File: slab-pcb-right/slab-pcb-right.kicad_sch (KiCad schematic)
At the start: 125 parts, among them J1 MagnetR, J2 MagnetL, J3 TRRS_R, J4 TRRS_L, J5 SSD1306, J6 Conn_01x06, Q1 MMBT3906, SW1 RotaryEncoder, U1 Seeeduino Xiao rp2040, U2 PCA9555PW, U3 PCA9555PW, U4 ADS1110, U5 SN74AHCT125PWR

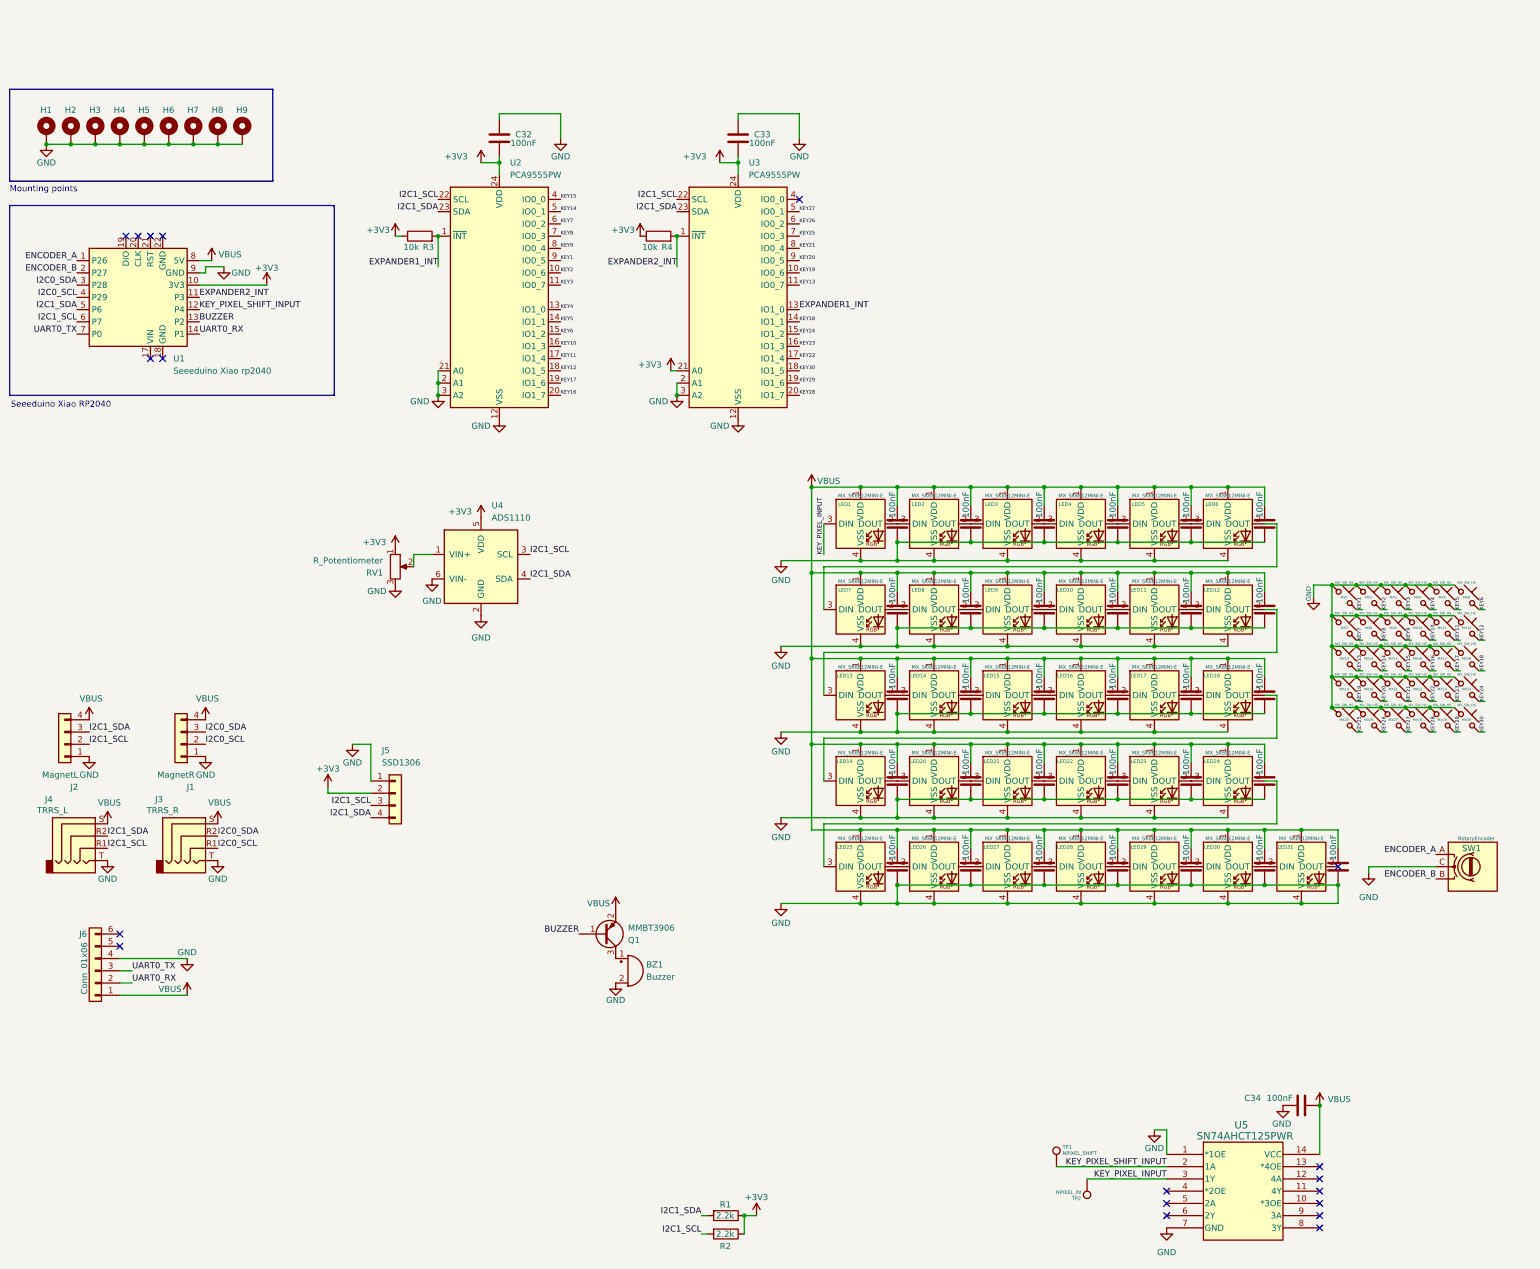
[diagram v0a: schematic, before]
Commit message: feat: start right board
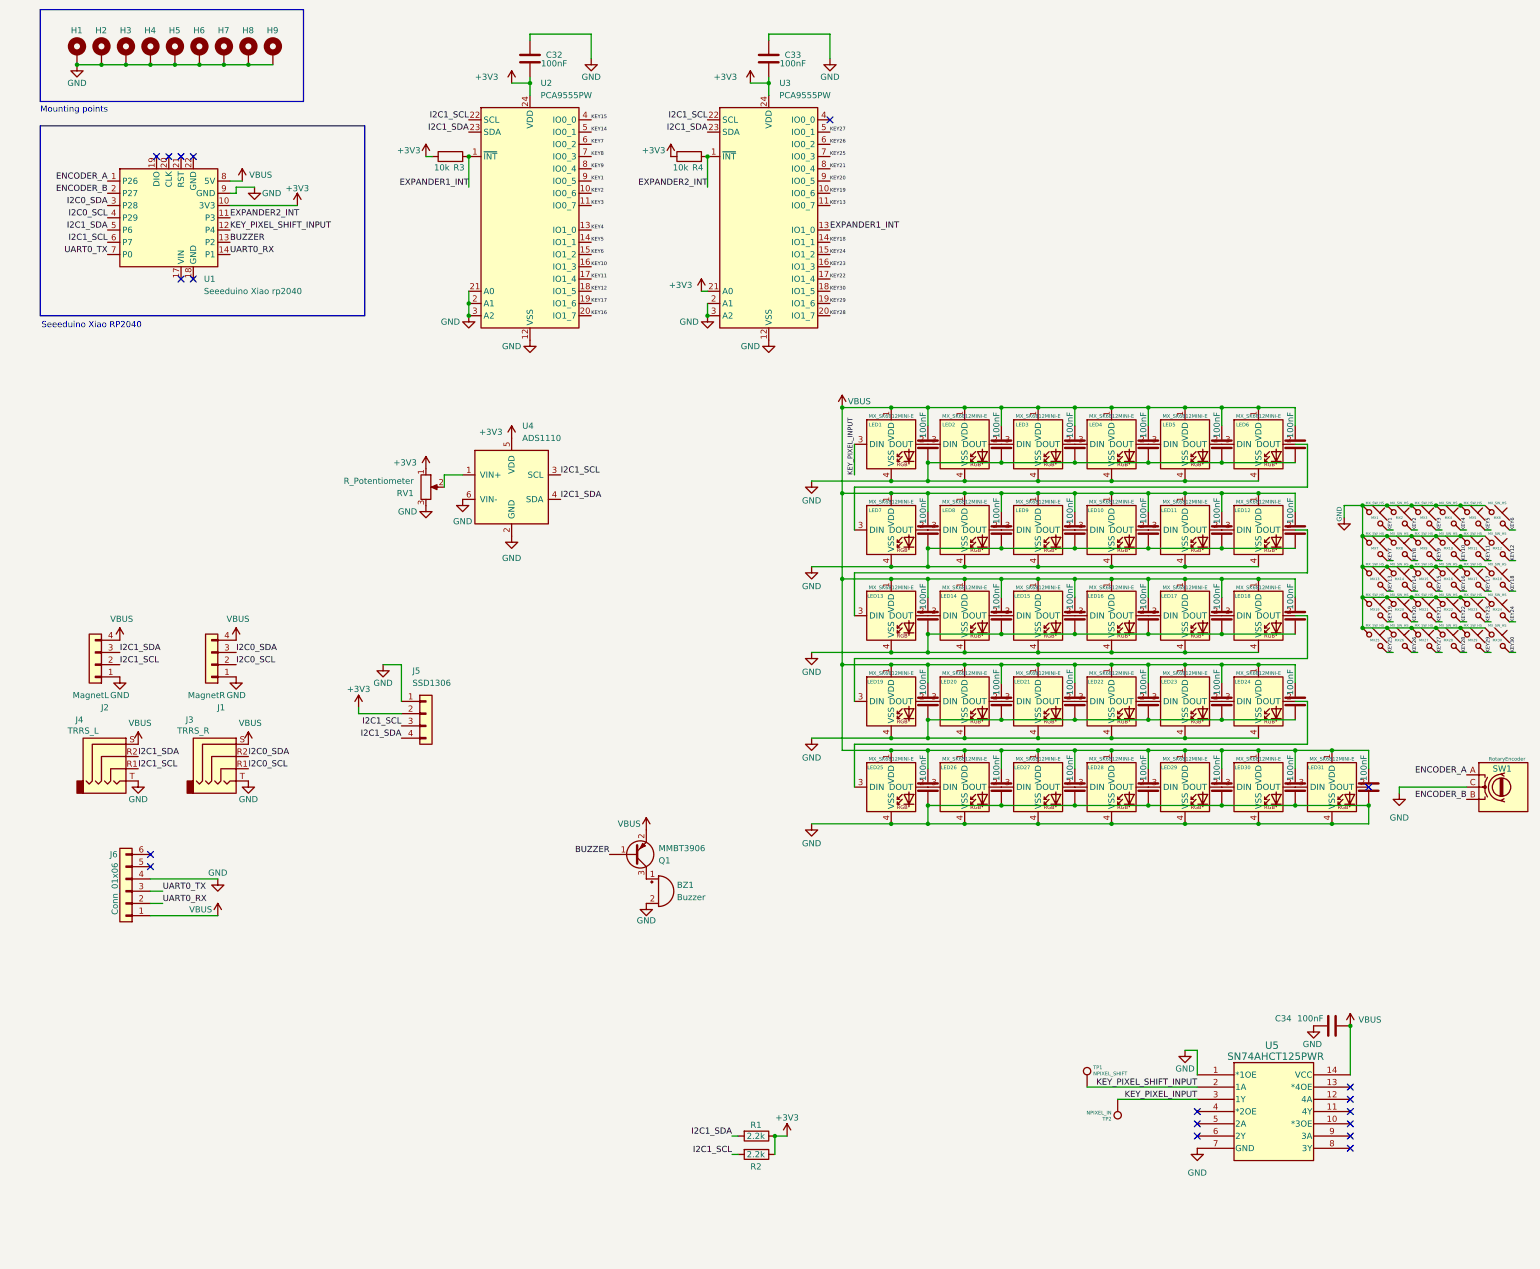
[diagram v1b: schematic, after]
